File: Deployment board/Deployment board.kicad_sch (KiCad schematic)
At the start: 28 parts, among them J1 Conn_01x04, J2 Conn_01x04, J3 Conn_01x02, J4 Conn_01x02, J5 Conn_01x02, J6 REMOVE BEFORE FLIGHT, M1 Motor_Servo, Q1 IRLR7843, Q2 IRLR7843, Q3 To be determined

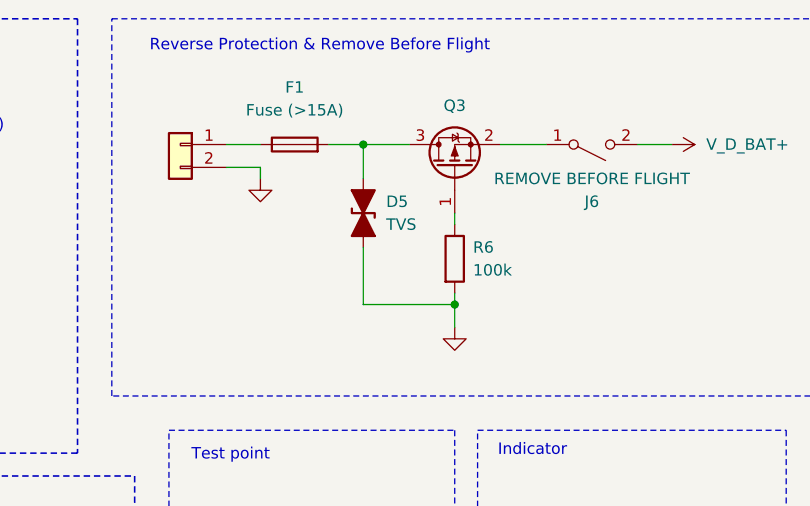
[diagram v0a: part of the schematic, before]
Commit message: jpush
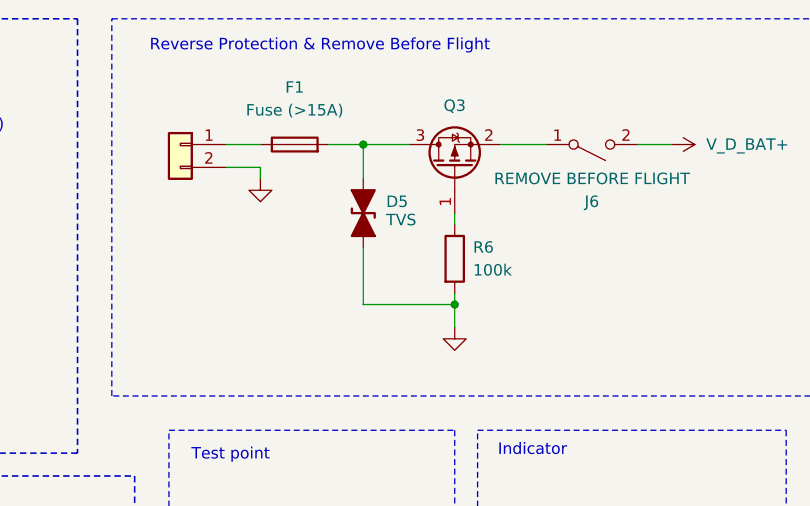
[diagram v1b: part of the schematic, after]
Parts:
- J1, J2: footprint Connector_PinSocket_2.54mm:PinSocket_1x04_P2.54mm_Horizontal -> Connector_PinSocket_2.54mm:PinSocket_1x04_P2.54mm_Vertical
- J3, J4: footprint Connector_PinSocket_2.54mm:PinSocket_1x02_P2.54mm_Horizontal -> Connector_PinSocket_2.54mm:PinSocket_1x02_P2.54mm_Vertical
- J5: footprint Connector_Wire:SolderWire-2sqmm_1x02_P7.8mm_D2mm_OD3.9mm -> Connector_JST:JST_EH_B2B-EH-A_1x02_P2.50mm_Vertical
- J6: footprint Connector_Wire:SolderWire-2sqmm_1x02_P7.8mm_D2mm_OD3.9mm -> Button_Switch_THT:SW_NKK_G1xJP
- M1: footprint Connector_PinHeader_2.54mm:PinHeader_1x03_P2.54mm_Horizontal -> Connector_PinHeader_2.54mm:PinHeader_1x03_P2.54mm_Vertical
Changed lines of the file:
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@@
 			)
 		)
-		(property "Footprint" "Connector_PinHeader_2.54mm:PinHeader_1x03_P2.54mm_Horizontal"
+		(property "Footprint" "Connector_PinHeader_2.54mm:PinHeader_1x03_P2.54mm_Vertical"
 			(at 74.93 49.276 0)
 			(effects
@@
 			)
 		)
-		(property "Footprint" "Connector_Wire:SolderWire-2sqmm_1x02_P7.8mm_D2mm_OD3.9mm"
+		(property "Footprint" "Button_Switch_THT:SW_NKK_G1xJP"
 			(at 176.53 30.48 0)
 			(effects
@@
 			)
 		)
-		(property "Footprint" "Connector_PinSocket_2.54mm:PinSocket_1x02_P2.54mm_Horizontal"
+		(property "Footprint" "Connector_PinSocket_2.54mm:PinSocket_1x02_P2.54mm_Vertical"
 			(at 102.87 86.36 0)
 			(effects
@@
 			)
 		)
-		(property "Footprint" "Connector_PinSocket_2.54mm:PinSocket_1x04_P2.54mm_Horizontal"
+		(property "Footprint" "Connector_PinSocket_2.54mm:PinSocket_1x04_P2.54mm_Vertical"
 			(at 71.12 144.78 0)
 			(effects
@@
 		)
 		(property "Value" "TVS"
-			(at 153.67 39.3699 90)
+			(at 153.67 38.862 90)
 			(effects
 				(font
@@
 			)
 		)
-		(property "Footprint" "Connector_PinSocket_2.54mm:PinSocket_1x02_P2.54mm_Horizontal"
+		(property "Footprint" "Connector_PinSocket_2.54mm:PinSocket_1x02_P2.54mm_Vertical"
 			(at 102.87 106.68 0)
 			(effects
@@
 			)
 		)
-		(property "Footprint" "Connector_Wire:SolderWire-2sqmm_1x02_P7.8mm_D2mm_OD3.9mm"
+		(property "Footprint" "Connector_JST:JST_EH_B2B-EH-A_1x02_P2.50mm_Vertical"
 			(at 130.81 30.48 0)
 			(effects
@@
 			)
 		)
-		(property "Footprint" "Connector_PinSocket_2.54mm:PinSocket_1x04_P2.54mm_Horizontal"
+		(property "Footprint" "Connector_PinSocket_2.54mm:PinSocket_1x04_P2.54mm_Vertical"
 			(at 25.4 144.78 0)
 			(effects

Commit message: jpush
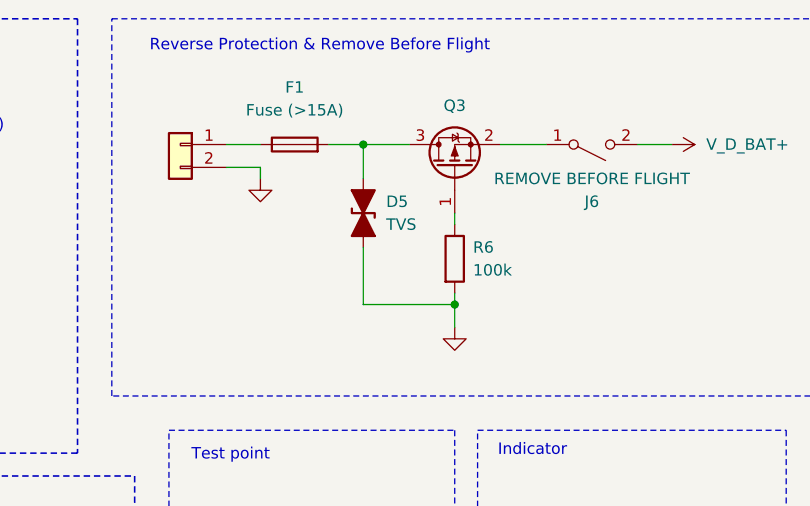
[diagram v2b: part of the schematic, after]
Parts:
- J1, J2: footprint Connector_PinSocket_2.54mm:PinSocket_1x04_P2.54mm_Vertical -> Connector_PinSocket_2.54mm:PinSocket_1x04_P2.54mm_Horizontal
- J3, J4: footprint Connector_PinSocket_2.54mm:PinSocket_1x02_P2.54mm_Vertical -> Connector_PinSocket_2.54mm:PinSocket_1x02_P2.54mm_Horizontal
- J5: footprint Connector_JST:JST_EH_B2B-EH-A_1x02_P2.50mm_Vertical -> Connector_Wire:SolderWire-2sqmm_1x02_P7.8mm_D2mm_OD3.9mm
- J6: footprint Button_Switch_THT:SW_NKK_G1xJP -> Connector_Wire:SolderWire-2sqmm_1x02_P7.8mm_D2mm_OD3.9mm
- M1: footprint Connector_PinHeader_2.54mm:PinHeader_1x03_P2.54mm_Vertical -> Connector_PinHeader_2.54mm:PinHeader_1x03_P2.54mm_Horizontal
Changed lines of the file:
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@@
 			)
 		)
-		(property "Footprint" "Connector_PinHeader_2.54mm:PinHeader_1x03_P2.54mm_Vertical"
+		(property "Footprint" "Connector_PinHeader_2.54mm:PinHeader_1x03_P2.54mm_Horizontal"
 			(at 74.93 49.276 0)
 			(effects
@@
 			)
 		)
-		(property "Footprint" "Button_Switch_THT:SW_NKK_G1xJP"
+		(property "Footprint" "Connector_Wire:SolderWire-2sqmm_1x02_P7.8mm_D2mm_OD3.9mm"
 			(at 176.53 30.48 0)
 			(effects
@@
 			)
 		)
-		(property "Footprint" "Connector_PinSocket_2.54mm:PinSocket_1x02_P2.54mm_Vertical"
+		(property "Footprint" "Connector_PinSocket_2.54mm:PinSocket_1x02_P2.54mm_Horizontal"
 			(at 102.87 86.36 0)
 			(effects
@@
 			)
 		)
-		(property "Footprint" "Connector_PinSocket_2.54mm:PinSocket_1x04_P2.54mm_Vertical"
+		(property "Footprint" "Connector_PinSocket_2.54mm:PinSocket_1x04_P2.54mm_Horizontal"
 			(at 71.12 144.78 0)
 			(effects
@@
 		)
 		(property "Value" "TVS"
-			(at 153.67 38.862 90)
+			(at 153.67 39.3699 90)
 			(effects
 				(font
@@
 			)
 		)
-		(property "Footprint" "Connector_PinSocket_2.54mm:PinSocket_1x02_P2.54mm_Vertical"
+		(property "Footprint" "Connector_PinSocket_2.54mm:PinSocket_1x02_P2.54mm_Horizontal"
 			(at 102.87 106.68 0)
 			(effects
@@
 			)
 		)
-		(property "Footprint" "Connector_JST:JST_EH_B2B-EH-A_1x02_P2.50mm_Vertical"
+		(property "Footprint" "Connector_Wire:SolderWire-2sqmm_1x02_P7.8mm_D2mm_OD3.9mm"
 			(at 130.81 30.48 0)
 			(effects
@@
 			)
 		)
-		(property "Footprint" "Connector_PinSocket_2.54mm:PinSocket_1x04_P2.54mm_Vertical"
+		(property "Footprint" "Connector_PinSocket_2.54mm:PinSocket_1x04_P2.54mm_Horizontal"
 			(at 25.4 144.78 0)
 			(effects
